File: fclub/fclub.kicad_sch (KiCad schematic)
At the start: 23 parts, among them SW1 SW_Push, SW10 SW_Push_45deg, SW2 SW_Push_45deg, SW3 SW_Push_45deg, SW4 SW_Push_45deg, SW5 SW_Push_45deg, SW6 SW_Push_45deg, SW7 SW_Push_45deg, SW8 SW_Push_45deg, SW9 SW_Push_45deg, U1 ATmega32U4-A, U2 STM32F042K4Tx, Y2 Crystal_GND24_Small

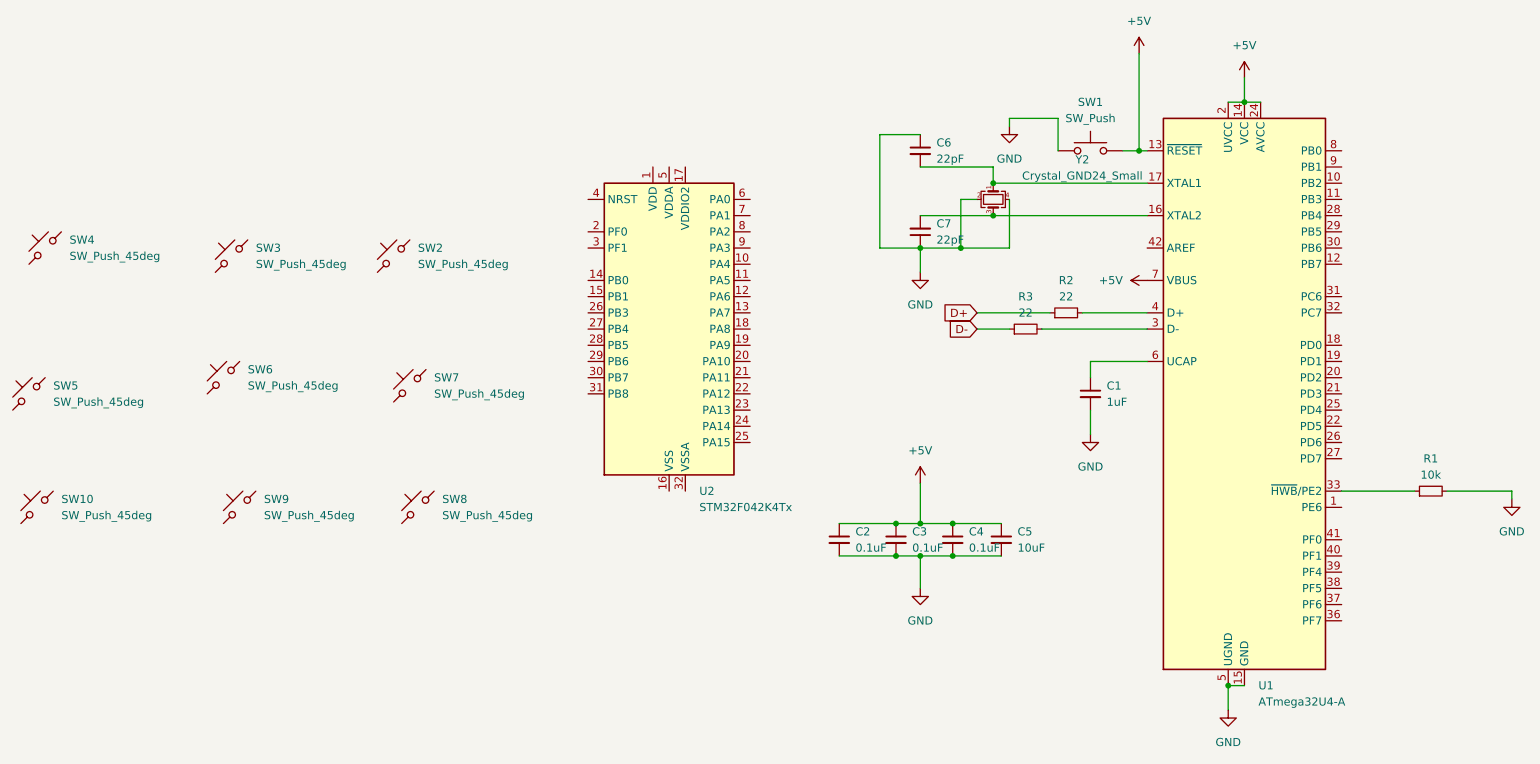
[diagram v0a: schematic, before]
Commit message: passage stm
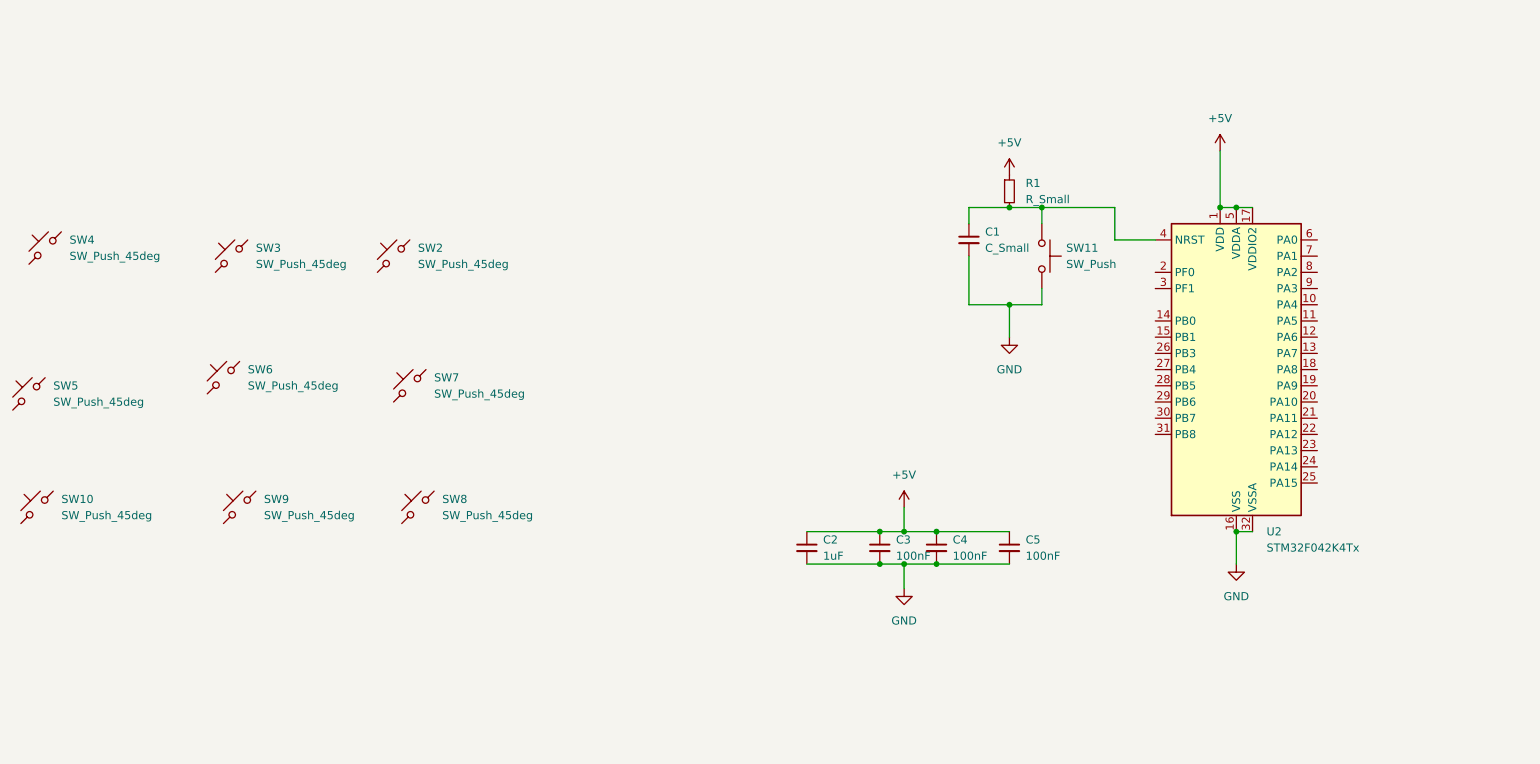
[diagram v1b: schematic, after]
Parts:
- removed C6, C7: 22pF, symbol Device:C_Small
- removed R2, R3: 22, symbol Device:R_Small
- removed SW1: SW_Push, symbol Switch:SW_Push
- removed U1: ATmega32U4-A, Package_QFP:TQFP-44_10x10mm_P0.8mm, symbol MCU_Microchip_ATmega:ATmega32U4-A
- removed Y2: Crystal_GND24_Small, symbol Device:Crystal_GND24_Small
- added SW11: SW_Push, symbol Switch:SW_Push
- C1: value 1uF -> C_Small
- C2: value 0.1uF -> 1uF
- C3, C4: value 0.1uF -> 100nF
- C5: value 10uF -> 100nF
- R1: value 10k -> R_Small
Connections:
- net +5V: now also R1.1, U2.1 (VDD), U2.17 (VDDIO2), U2.5 (VDDA)
- net GND: now also U2.16 (VSS), U2.32 (VSSA), SW11.2; no longer R1.2
- net at C1.1: now also R1.2, U2.4 (NRST), SW11.1
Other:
- moved on the sheet: U2
